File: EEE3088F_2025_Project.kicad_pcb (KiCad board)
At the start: 2 copper layers, 81 x 53.5 mm, 66 parts, among them J1 Conn_02x16_Odd_Even, J2 USB_C_Receptacle_PowerOnly_6P, J3 Conn_01x02, Q2 NMOS, SW1 SW_SPDT, U1 HR8833, U10 INA219AIDCNR, U11 AP2171WG-7, U2 HR8833, U4 AP2112K-3.3, U5 TPS613222ADBVR, U6 HUSB237-AA001-DN06R, U7 AP2171WG-7, U8 TP4056-42-ESOP8, U9 CJ78L05

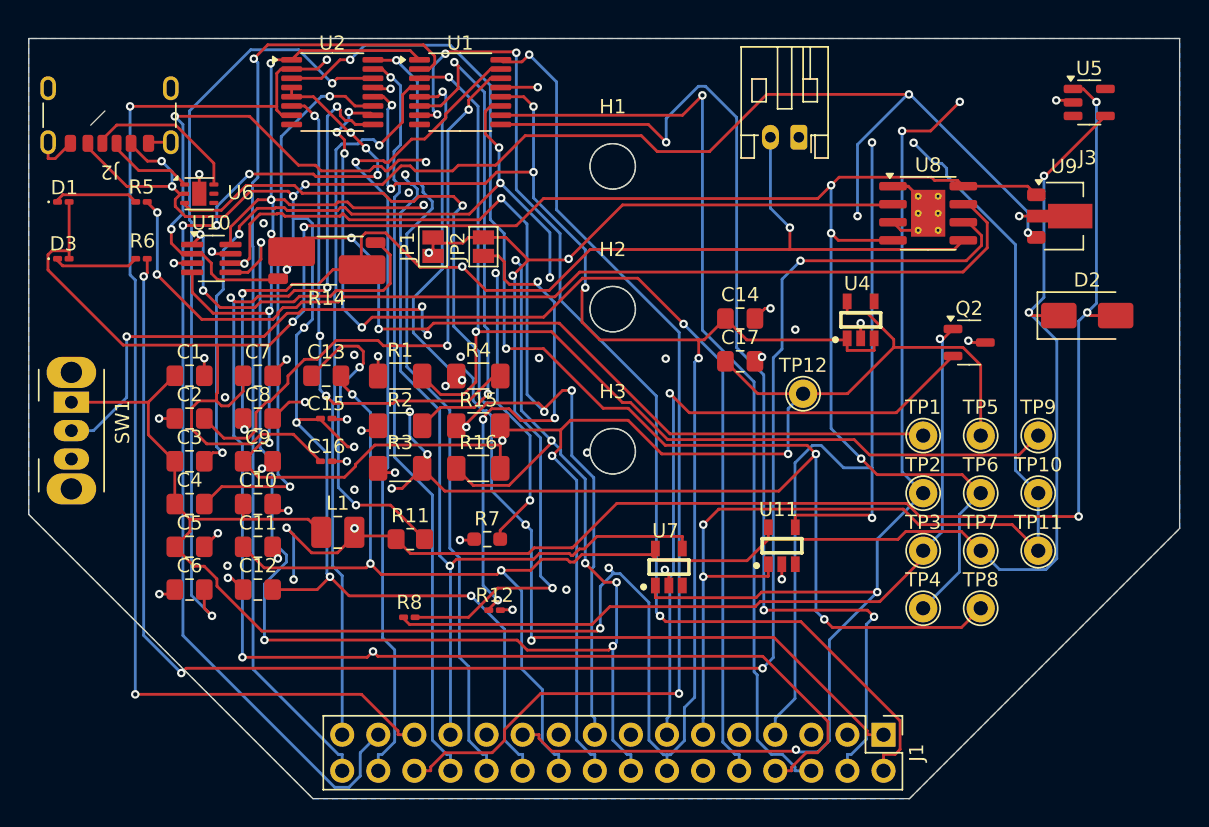
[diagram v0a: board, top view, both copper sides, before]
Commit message: added routing
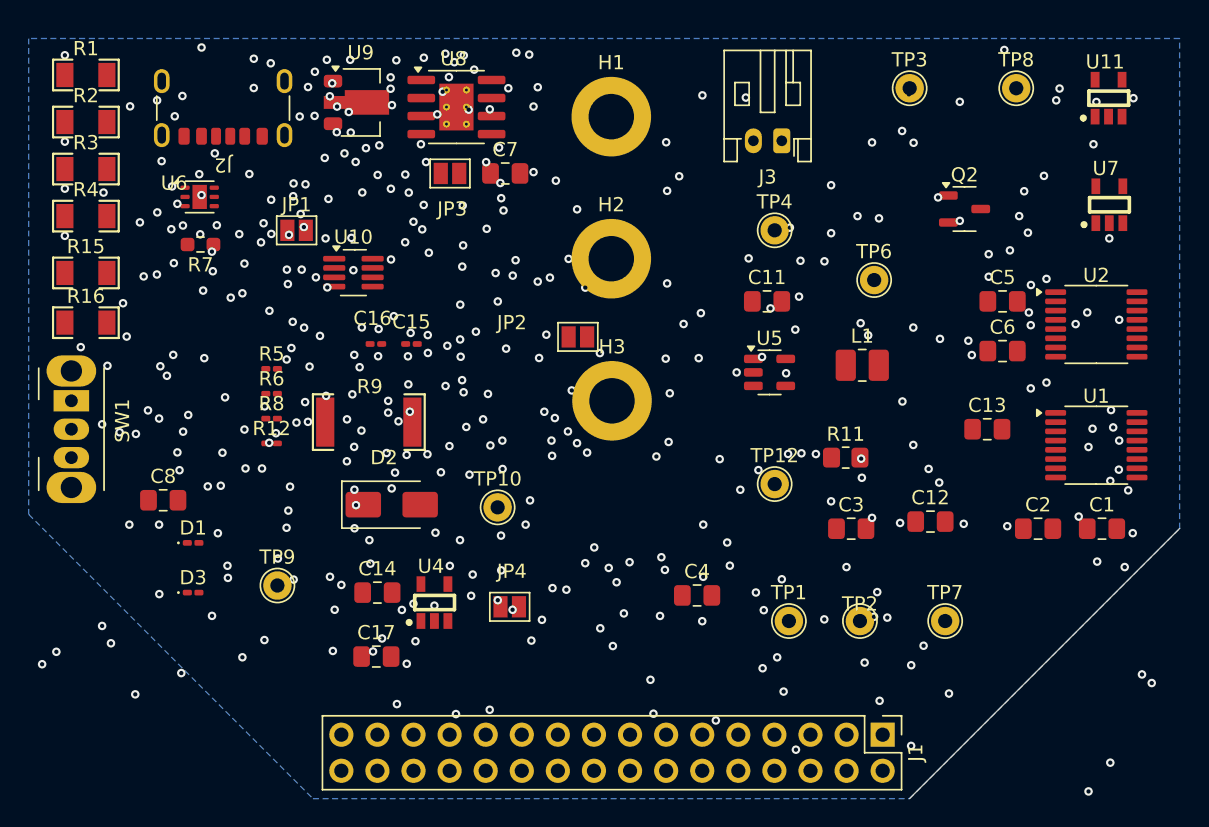
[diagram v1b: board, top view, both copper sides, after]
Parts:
- removed C10, C9: 10u, Capacitor_SMD:C_0805_2012Metric_Pad1.18x1.45mm_HandSolder
- removed R14: 3m, Resistor_SMD:R_Shunt_Vishay_WSK2512_6332Metric_T2.21mm
- removed TP11, TP5: TestPoint, TestPoint:TestPoint_THTPad_D2.0mm_Drill1.0mm
- added JP3: SolderJumper_2_Open, Jumper:SolderJumper-2_P1.3mm_Open_Pad1.0x1.5mm, F.Cu at (73.2, 85.0)
- added JP4: SolderJumper_2_Open, Jumper:SolderJumper-2_P1.3mm_Open_Pad1.0x1.5mm, F.Cu at (77.3, 115.5)
- added R9: 3m, Library:R2512, F.Cu at (67.4, 102.5)
- H1, H2, H3: footprint MountingHole:MountingHole_3.2mm_M3 -> MountingHole:MountingHole_3.2mm_M3_DIN965_Pad
- R1, R15, R16, R2, R3, R4: footprint Resistor_SMD:R_1206_3216Metric_Pad1.30x1.75mm_HandSolder -> Library:R1206
- moved C1 65.1 mm to (119.0, 110.0)
- moved C2 60.2 mm to (114.5, 110.0)
- moved C5 59.8 mm to (112.0, 94.0)
- moved C6 59.6 mm to (112.0, 97.5)
- moved U2 56.2 mm to (118.6, 95.6)
- moved TP9 54.6 mm to (61.0, 114.0)
- moved U1 51.2 mm to (118.6, 104.1)
- moved D2 50.7 mm to (69.0, 108.3)
- moved U9 50.1 mm to (66.9, 80.0)
- moved C12 47.6 mm to (107.0, 109.5)
- moved C3 46.8 mm to (101.4, 110.0)
- moved C13 46.7 mm to (111.0, 103.0)
- moved U7 40.1 mm to (119.6, 87.2)
- moved C11 39.8 mm to (95.5, 94.0)
- moved U11 39.0 mm to (119.5, 79.7)
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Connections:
- C16 pad 1: /5V -> Net-(JP3-B)
- C17 pad 1: /3V3 Out -> Net-(JP4-B)
- C8 pad 1: /Vbat -> /IN+
- J3 pad 2: /Vbat -> /IN+
- SW1 pad 2: Net-(SW1-B) -> /IN-
- TP1 pad 1: Net-(SW1-B) -> /IN-
- TP12 pad 1: /3V3 Out -> Net-(JP4-B)
- TP6 pad 1: /5V -> Net-(JP3-B)
- U4 pad 5: /3V3 Out -> Net-(JP4-B)
- U8 pad 5: /Vbat -> /IN+
- U9 pad 1: /5V -> Net-(JP3-B)
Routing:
- net /Battery: track 175.8 -> 0.00 mm, vias 8 -> 11
- net /3V3 Out: track 169.9 -> 0.00 mm, vias 10 -> 5
- net /HV: track 162.7 -> 0.00 mm, vias 13 -> 16
- net /5V: track 152.7 -> 0.00 mm, vias 5 -> 10
- net /5V Out: track 129.6 -> 0.00 mm, vias 5 -> 9
- net Net-(U2-AISEN): track 120.5 -> 0.00 mm, vias 7 -> 6
- net Net-(U8-~{STDBY}): track 116.8 -> 0.00 mm, vias 4 -> 7
- net /I2C1_SCL: track 106.9 -> 0.00 mm, vias 7 -> 3
- net /MOTOR4_CTRL1: track 98.9 -> 0.00 mm
- net Net-(D2-A): track 97.5 -> 0.00 mm, vias 6 -> 2
- net /EXT_LOAD1_OUT: track 90.5 -> 0.00 mm, vias 4 -> 7
- net Net-(SW1-B): track 87.0 -> 0.00 mm, vias 5 -> 0
- net /MOTOR3_A_OUT: track 80.5 -> 0.00 mm, vias 3 -> 4
- net /Motor2_A_OUT: track 79.4 -> 0.00 mm, vias 4 -> 8
- net /EXT_LOAD2_OUT: track 78.2 -> 0.00 mm, vias 3 -> 4
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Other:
- board size 81 x 53.5 mm -> 19 x 19 mm
